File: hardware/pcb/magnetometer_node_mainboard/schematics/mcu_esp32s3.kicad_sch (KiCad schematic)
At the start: 1 part, among them U7 ESP32-S3-WROOM-1

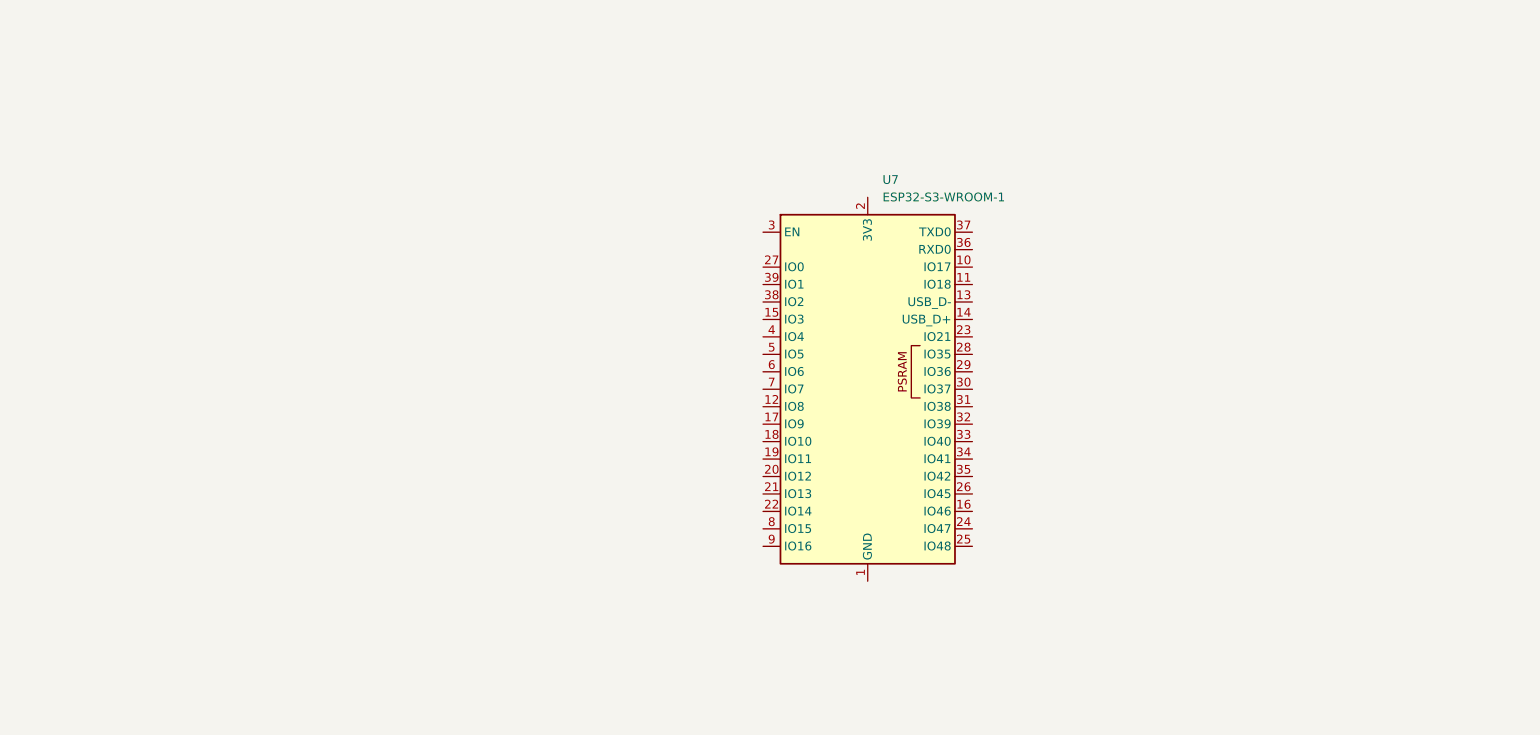
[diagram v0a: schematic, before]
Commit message: first code for the v1
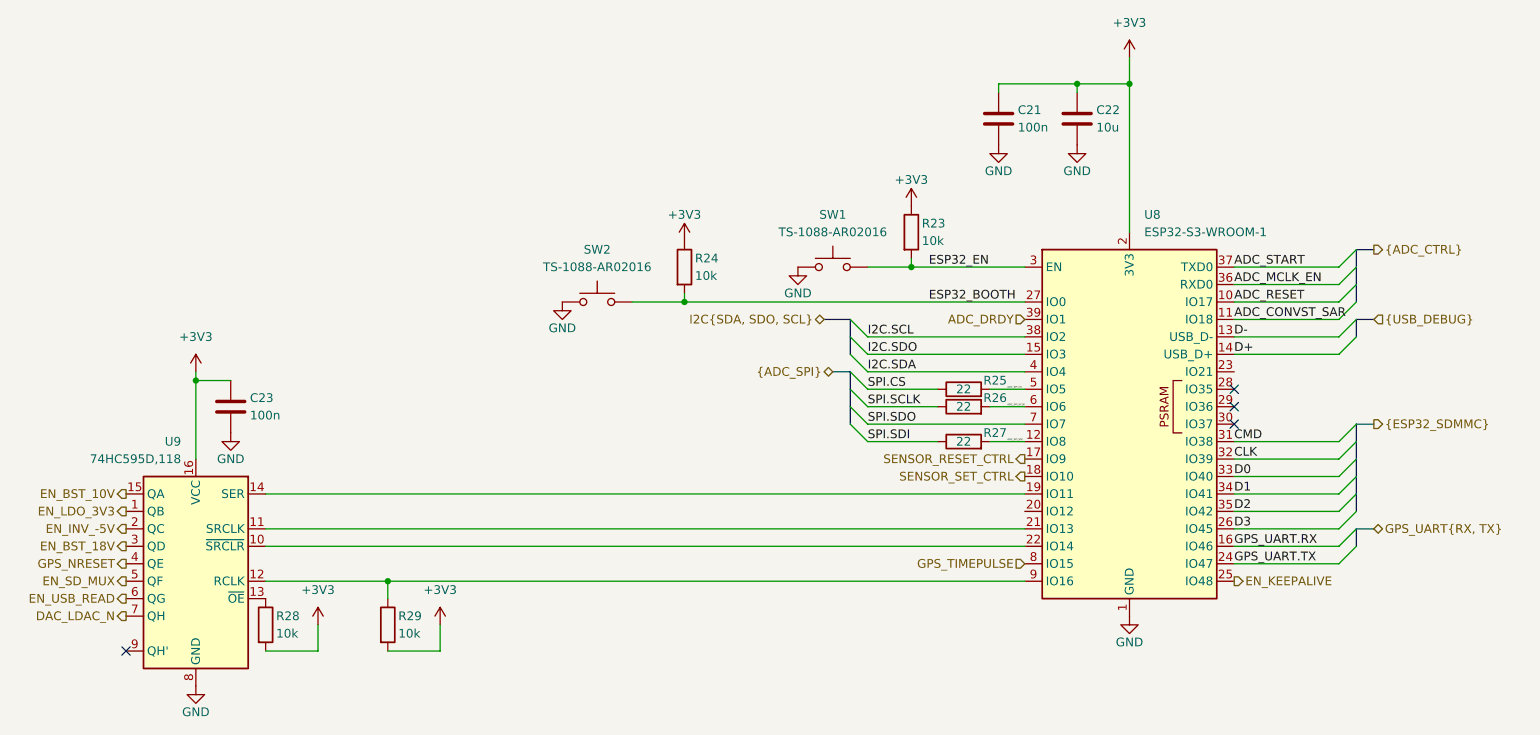
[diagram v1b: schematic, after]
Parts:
- added C21, C23: 100n, Capacitor_SMD:C_0603_1608Metric, symbol Device:C
- added C22: 10u, Capacitor_SMD:C_0805_2012Metric, symbol Device:C
- added R23, R24, R28, R29: 10k, Resistor_SMD:R_0603_1608Metric, symbol Device:R
- added R25, R26, R27: 22, Resistor_SMD:R_0603_1608Metric, symbol Device:R
- added SW1, SW2: TS-1088-AR02016, magnode_footprints:TS-1088-AR02016, symbol Switch:SW_Push
- added U9: 74HC595D,118, Package_SO:SOIC-16_3.9x9.9mm_P1.27mm, symbol 74xx:74HC595
- renumbered U7 to U8
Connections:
- net GND: now reaches U8.1 (GND), U8.40 (GND), U8.41 (GND)
- net GND: now also C21.2, C22.2, C23.2, SW1.1, SW2.1, U9.8 (GND)
- net ADC_RESET: now reaches U8.10 (IO17)
- net ADC_CONVST_SAR: now reaches U8.11 (IO18)
- net ADC_SPI_SDI: now reaches U8.12 (IO8)
- net ADC_SPI_SDI: now also R27.2
- net D-: now reaches U8.13 (USB_D-)
- net D+: now reaches U8.14 (USB_D+)
- net I2C.SDO: now reaches U8.15 (IO3)
- net GPS_UART.RX: now reaches U8.16 (IO46)
- net SENSOR_RESET_CTRL: now reaches U8.17 (IO9)
- net SENSOR_SET_CTRL: now reaches U8.18 (IO10)
- net at U8.19 (IO11): now also U9.14 (SER)
- net +3V3: now reaches U8.2 (3V3)
- net +3V3: now also C21.1, C22.1, C23.1, R23.1, R24.1, R28.2, R29.2, U9.16 (VCC)
- net at U8.21 (IO13): now also U9.11 (SRCLK)
- net at U8.22 (IO14): now also U9.10 (~{SRCLR})
- net GPS_UART.TX: now reaches U8.24 (IO47)
- net EN_KEEPALIVE: now reaches U8.25 (IO48)
- net D3: now reaches U8.26 (IO45)
- net ESP32_BOOTH: now reaches U8.27 (IO0)
- net ESP32_BOOTH: now also R24.2, SW2.2
- net ESP32_EN: now reaches U8.3 (EN)
- net ESP32_EN: now also R23.2, SW1.2
- net CMD: now reaches U8.31 (IO38)
- net CLK: now reaches U8.32 (IO39)
- net D0: now reaches U8.33 (IO40)
- net D1: now reaches U8.34 (IO41)
- net D2: now reaches U8.35 (IO42)
- net ADC_MCLK_EN: now reaches U8.36 (RXD0)
- net ADC_START: now reaches U8.37 (TXD0)
- net I2C.SCL: now reaches U8.38 (IO2)
- net ADC_DRDY: now reaches U8.39 (IO1)
- net I2C.SDA: now reaches U8.4 (IO4)
- net ADC_SPI_CS: now reaches U8.5 (IO5)
- net ADC_SPI_CS: now also R25.2
- net ADC_SPI_SCLK: now reaches U8.6 (IO6)
- net ADC_SPI_SCLK: now also R26.2
- net SPI.SDO: now reaches U8.7 (IO7)
- net GPS_TIMEPULSE: now reaches U8.8 (IO15)
- net at U8.9 (IO16): now also R29.1, U9.12 (RCLK)
- new net: R28.1, U9.13 (~{OE})
- new net DAC_LDAC_N: U9.7 (QH)
- new net EN_BST_10V: U9.15 (QA)
- new net EN_BST_18V: U9.3 (QD)
- new net EN_INV_-5V: U9.2 (QC)
- new net EN_LDO_3V3: U9.1 (QB)
- new net EN_SD_MUX: U9.5 (QF)
- new net EN_USB_READ: U9.6 (QG)
- new net GPS_NRESET: U9.4 (QE)
- new net SPI.CS: R25.1
- new net SPI.SCLK: R26.1
- new net SPI.SDI: R27.1
- no-connect marks 0 -> 4
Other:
- moved on the sheet: U8
